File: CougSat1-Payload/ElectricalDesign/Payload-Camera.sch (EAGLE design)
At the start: 41 parts, among them J1 CougSat Card, U1 AD7291, U2 AD8515, U3 AD8616, U4 AD8515, U5 CD74HC4040M

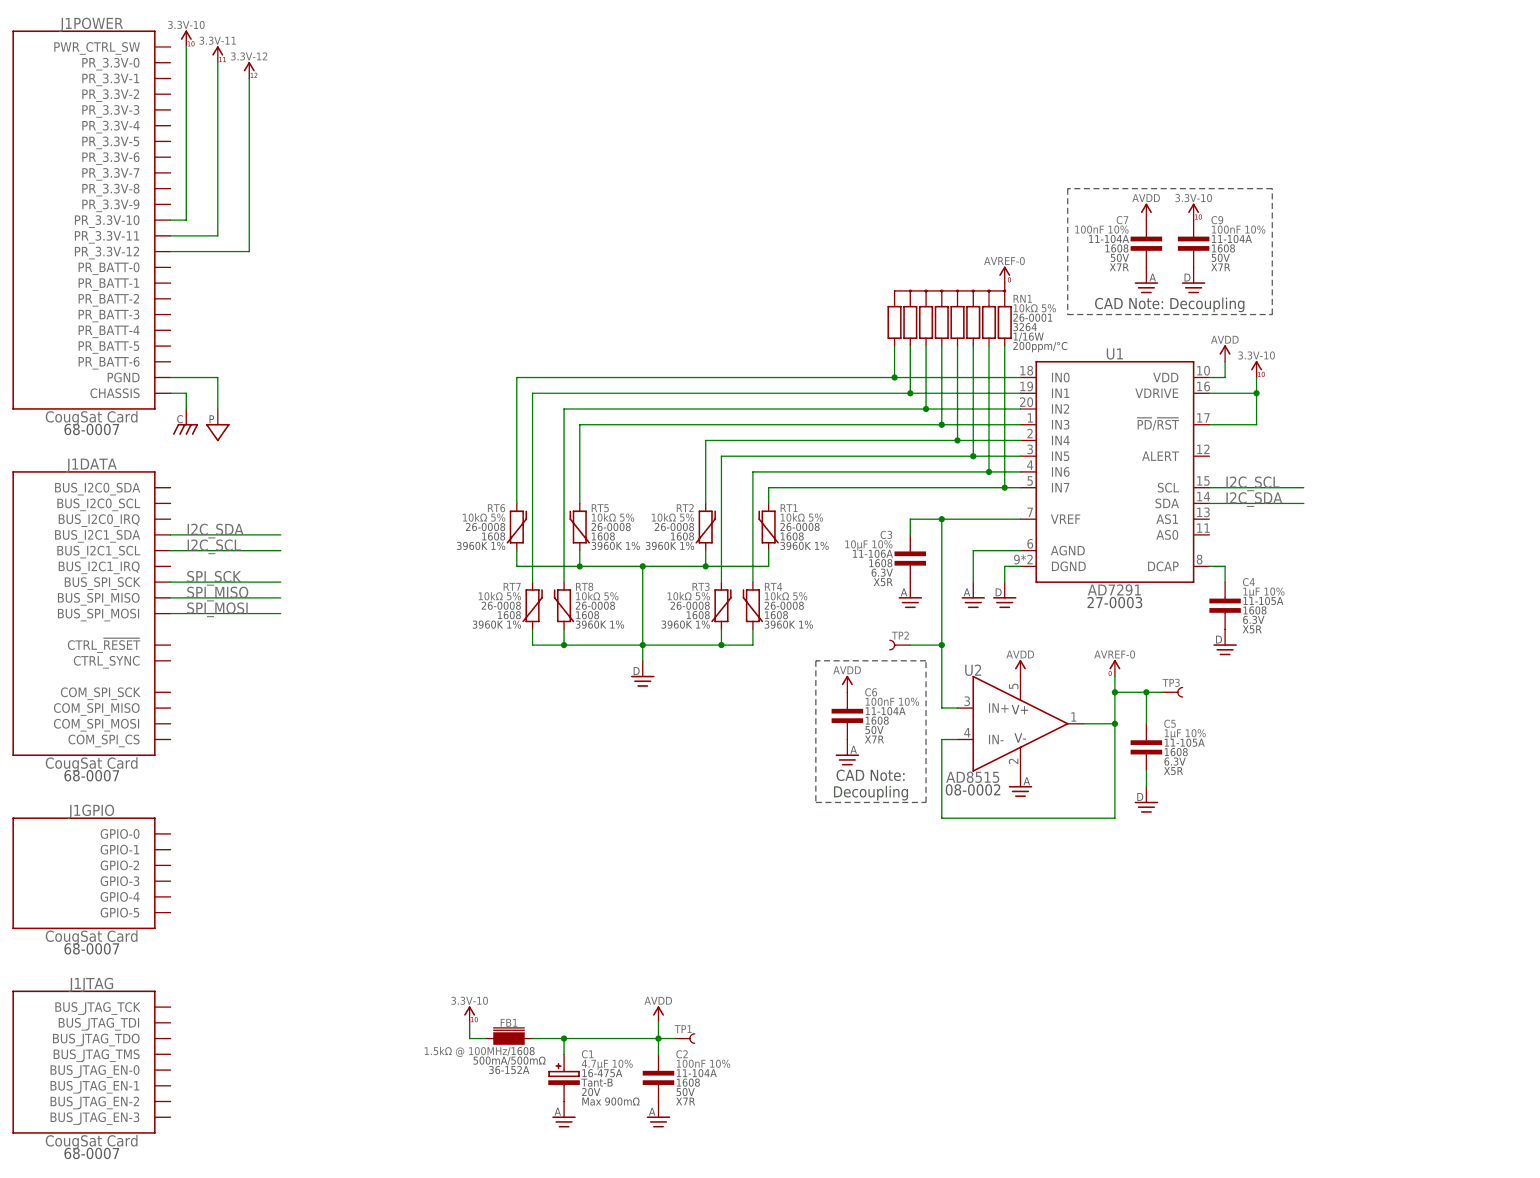
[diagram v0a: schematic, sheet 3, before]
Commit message: Created design document
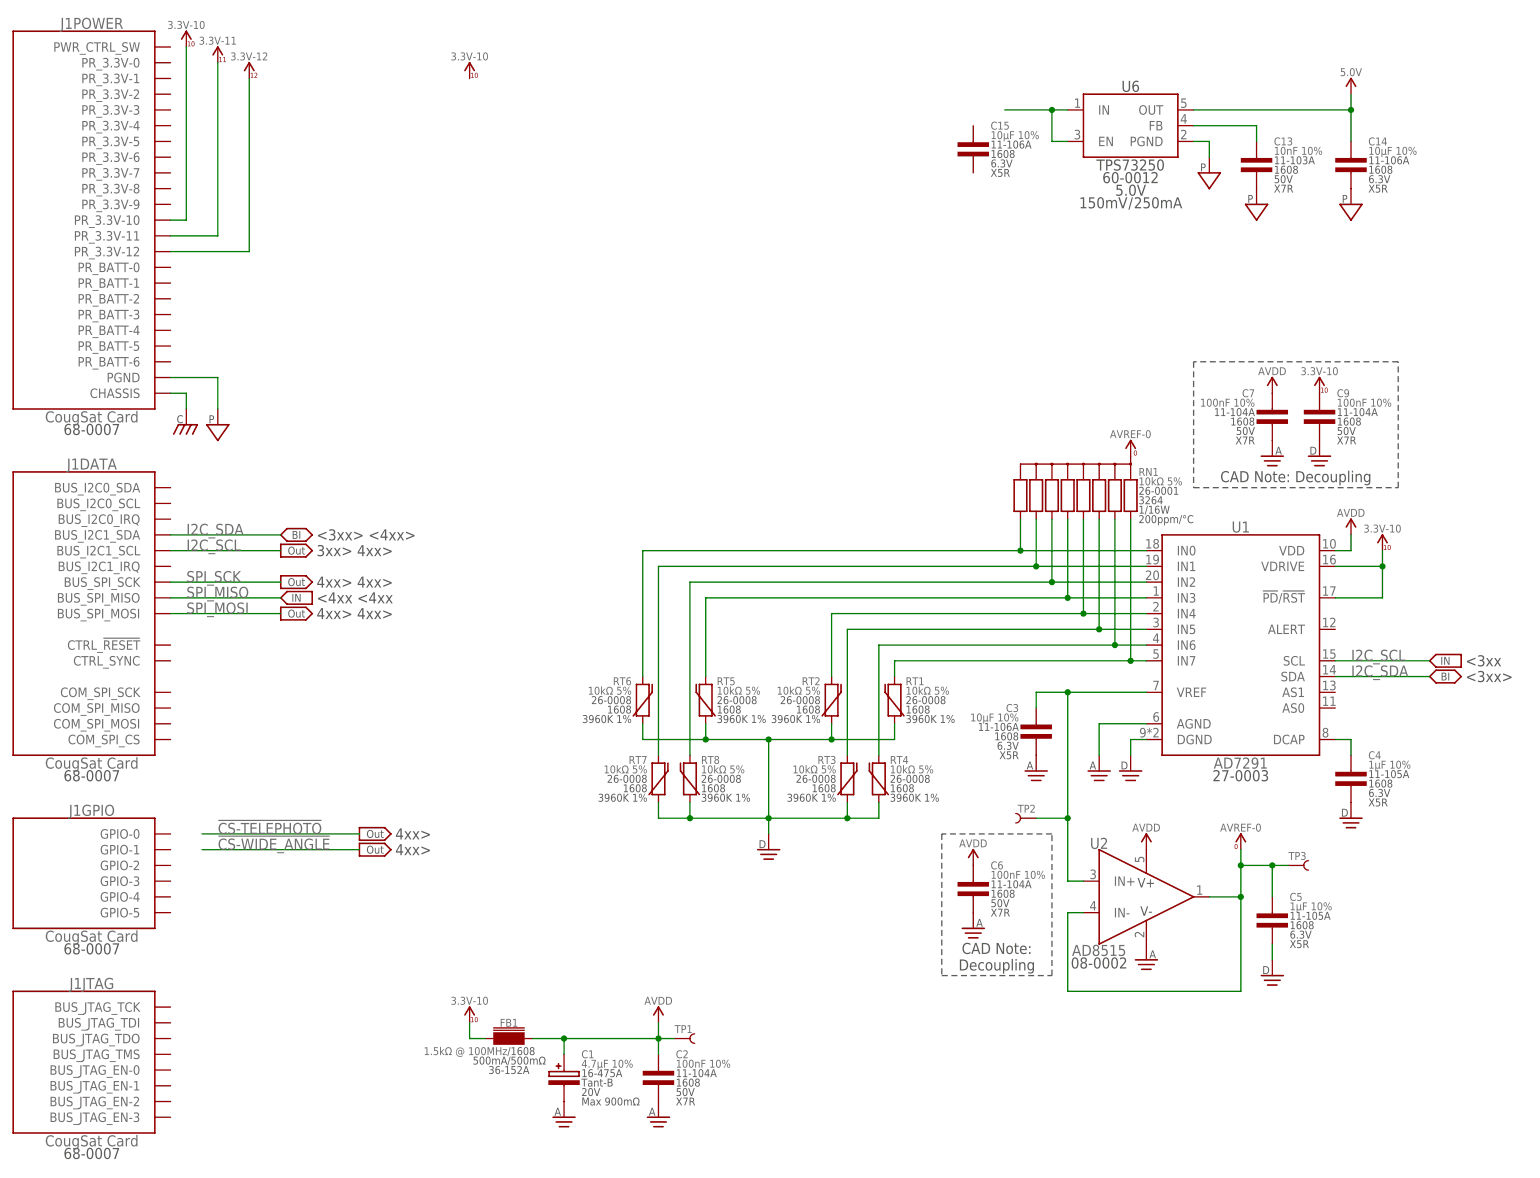
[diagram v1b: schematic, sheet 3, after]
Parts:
- added C13: 10nF 10%, CougsInSpace-Capacitors:CAP-V-10NF-1608
- added C14, C15: 10µF 10%, CougsInSpace-Capacitors:CAP-V-10UF-1608
- added U6: TPS73250, CougsInSpace-IC-Power:LDO-FB-5.0-SOT23-5
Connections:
- new net N$17: U4.OUT, U5.IN
- new net N$18: U6.EN, U6.IN
- new net N$19: C13.1, U6.FB
- net 3.3V_10: now also U5.VCC
- net 5.0V: now also C14.1, U6.OUT
- net DGND: now also U5.DGND
- net PGND: now also C13.2, C14.2, U6.PGND
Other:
- note added: "3xx>"
- note added: "3xx> 4xx>"
- note added: "4xx>"
- note added: "4xx> 4xx>"
- note added: "<3xx"
- note added: "<3xx>"
- note added: "<3xx> <4xx>"
- note added: "<4xx <4xx"
- moved on the sheet: C10, C11, C12, C3, C4, C5, C6, C7, C8, C9, D1, R1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
